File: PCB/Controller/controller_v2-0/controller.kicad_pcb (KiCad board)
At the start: 2 copper layers, 70 x 55 mm, 22 parts, among them J1 16-Pin LCD, J2 PWR, J3 Inter Board, J4 Conn_01x19, J5 Conn_01x19, U1 ESP32-DEVKITC-32E, U2 AMS1117-5.0, U3 SP3485EN, U4 AMS1117-3.3

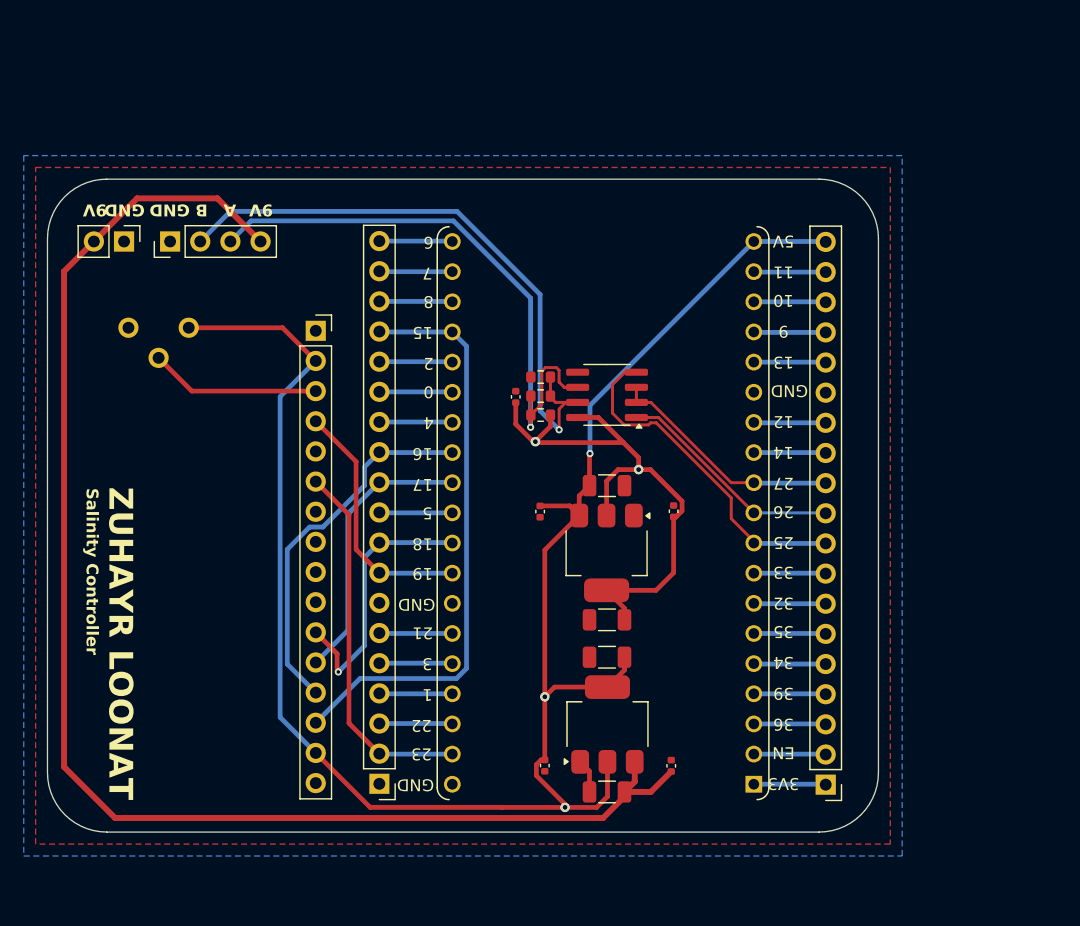
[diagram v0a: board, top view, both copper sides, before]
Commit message: Gerbers and BOMS
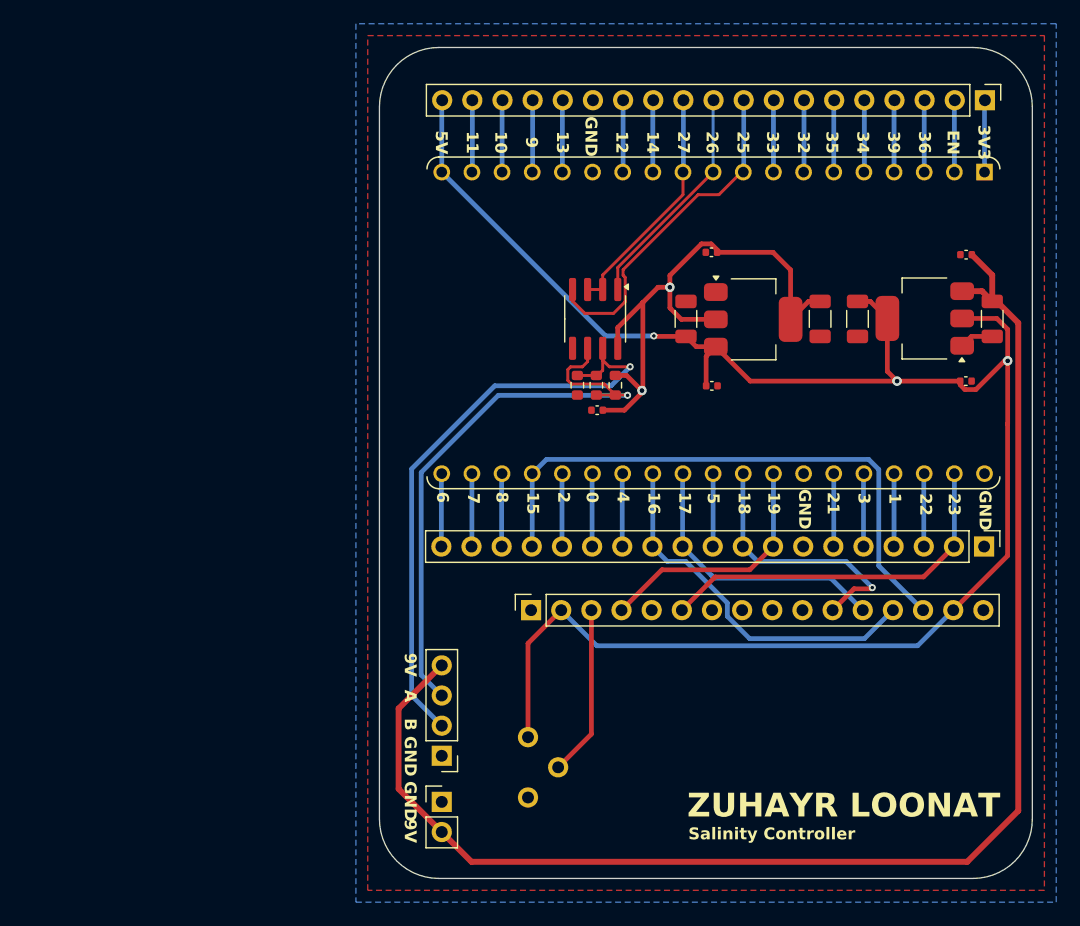
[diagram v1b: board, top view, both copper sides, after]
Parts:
- moved J4 59.2 mm to (219.0, 33.3), turned to -90 degrees
- moved J5 54.7 mm to (218.9, 70.9), turned to -90 degrees
- moved J2 54.3 mm to (173.2, 92.4), turned to 0 degrees
- moved RV1 51.8 mm to (183.0, 92.1), turned to 180 degrees
- moved C3 51.4 mm to (219.6, 51.8), turned to -90 degrees
- moved C2 49.7 mm to (217.4, 46.3), turned to 180 degrees
- moved J3 49.0 mm to (173.2, 88.6), turned to 180 degrees
- moved C5 48.0 mm to (217.4, 57.0), turned to 0 degrees
- moved U2 43.4 mm to (213.9, 51.7), turned to 180 degrees
- moved C7 35.5 mm to (208.2, 51.8), turned to -90 degrees
- moved C8 31.1 mm to (205.1, 51.8), turned to -90 degrees
- moved J1 29.7 mm to (180.7, 76.3), turned to 90 degrees
- moved U4 23.2 mm to (199.4, 51.8), turned to 0 degrees
- moved C9 22.0 mm to (195.9, 46.1), turned to 180 degrees
- moved U1 18.5 mm to (196.1, 52.1), turned to -90 degrees
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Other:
- board size 70 x 55 mm -> 55 x 70 mm
